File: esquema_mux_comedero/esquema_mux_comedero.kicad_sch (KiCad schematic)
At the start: 7 parts

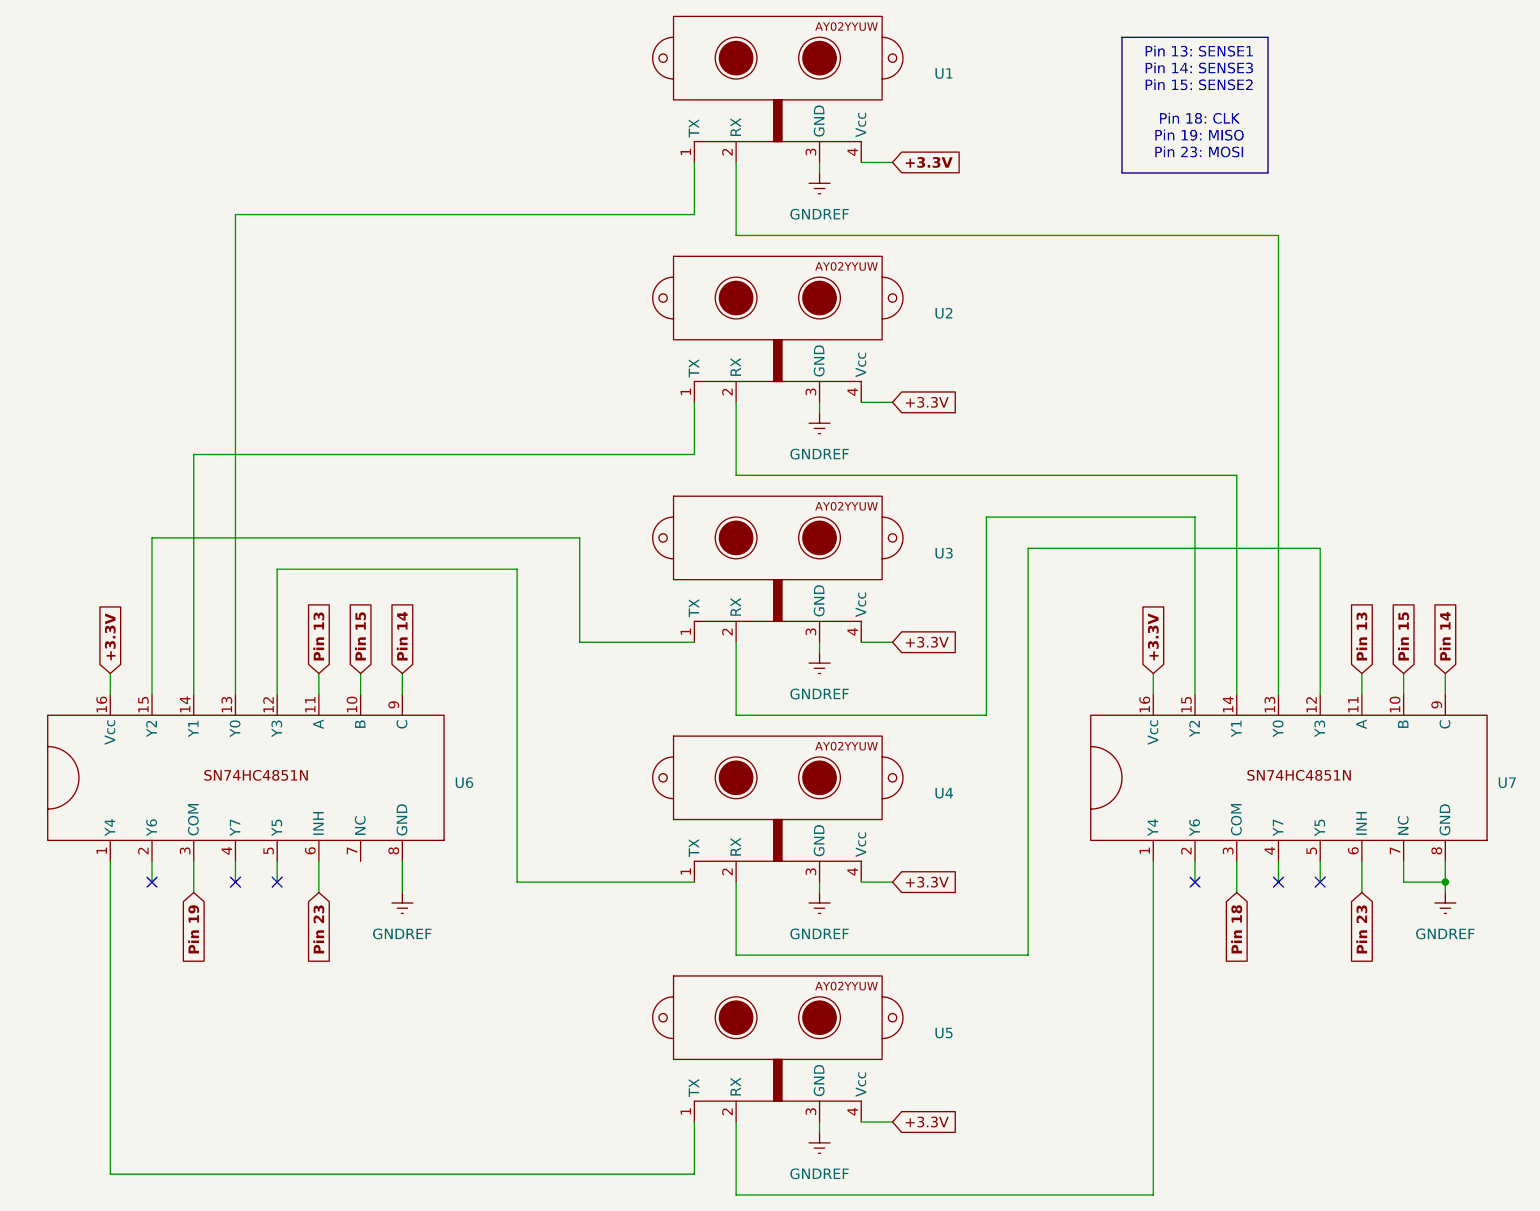
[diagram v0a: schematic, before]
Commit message: opt
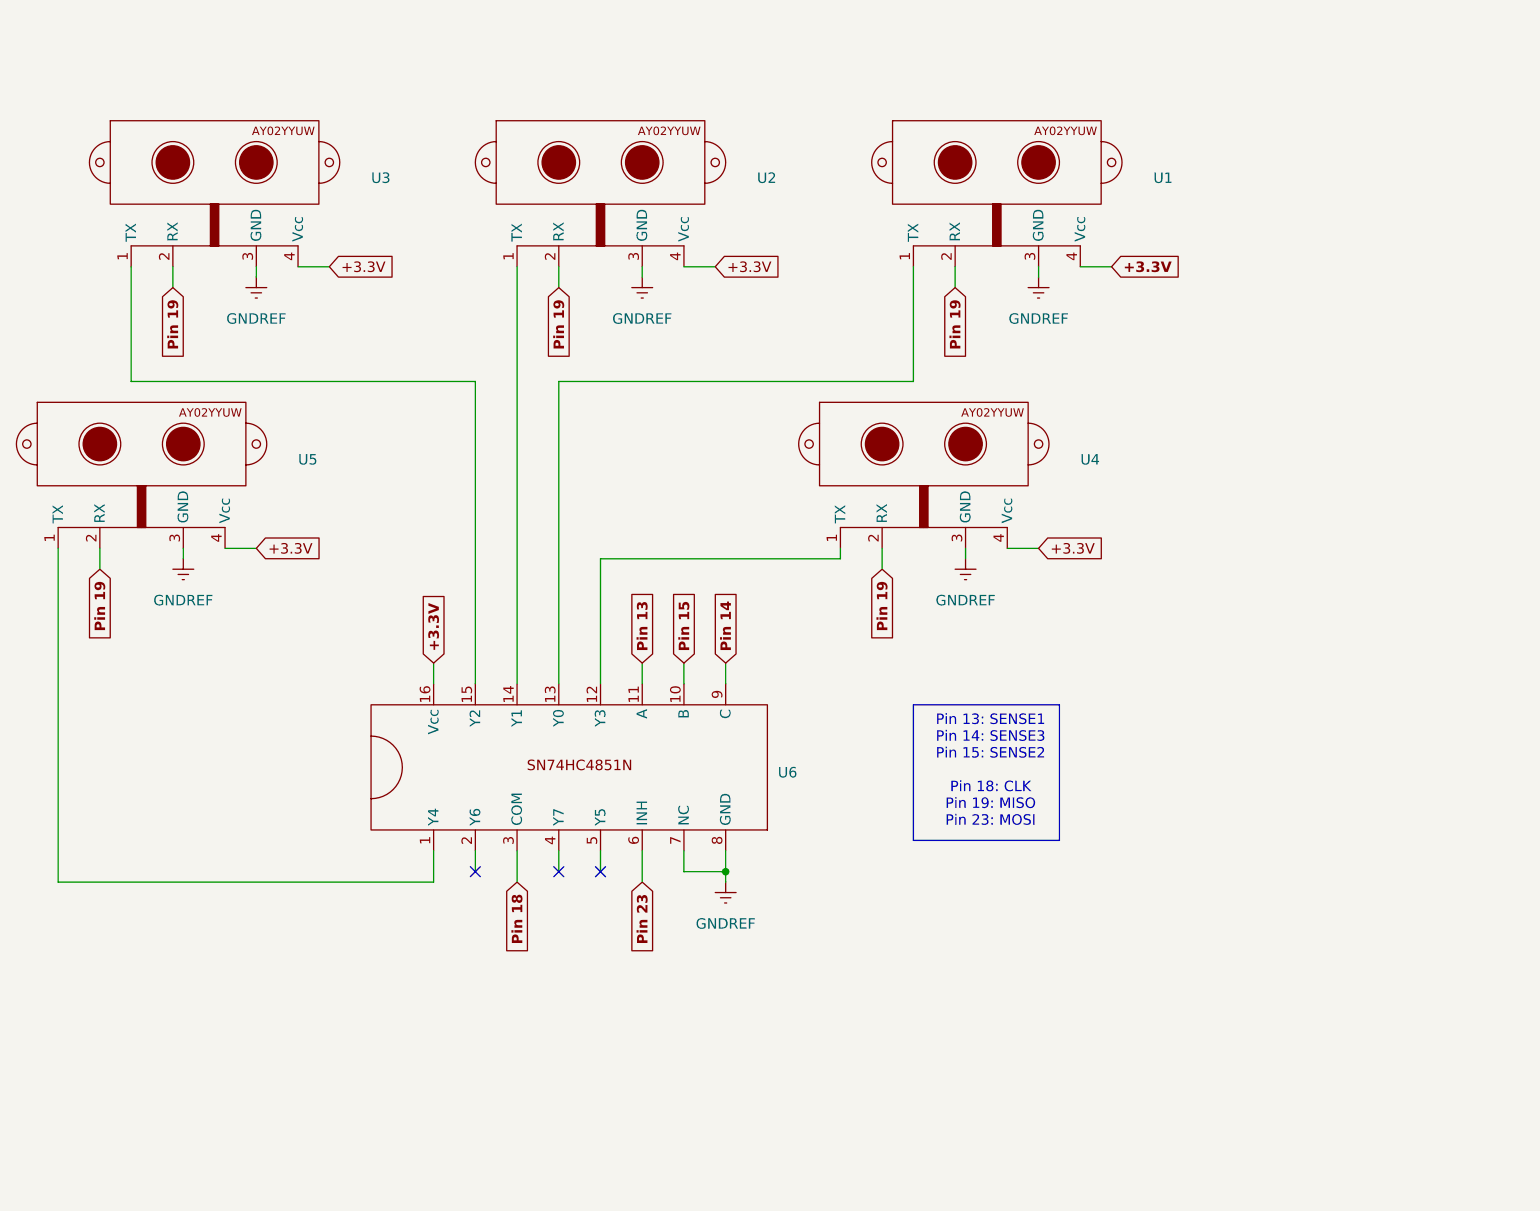
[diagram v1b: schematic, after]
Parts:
- removed U7: ~, symbol Mensoft_Carmen:SN74HC4851N
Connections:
- net GNDREF: now also U6.7 (NC)
- net Pin 18: now also U6.3 (COM)
- net Pin 19: now also U1.2 (RX), U2.2 (RX), U3.2 (RX), U4.2 (RX), U5.2 (RX); no longer U6.3 (COM)
- no-connect marks 6 -> 3
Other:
- moved on the sheet: U1, U2, U3, U4, U5, U6
